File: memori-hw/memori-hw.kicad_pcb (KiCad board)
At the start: 4 copper layers, 2 parts, among them J1 WeAct Studio 2.9" E-Paper Dis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, J2 Seeed Studio Xiao ESP32-C3

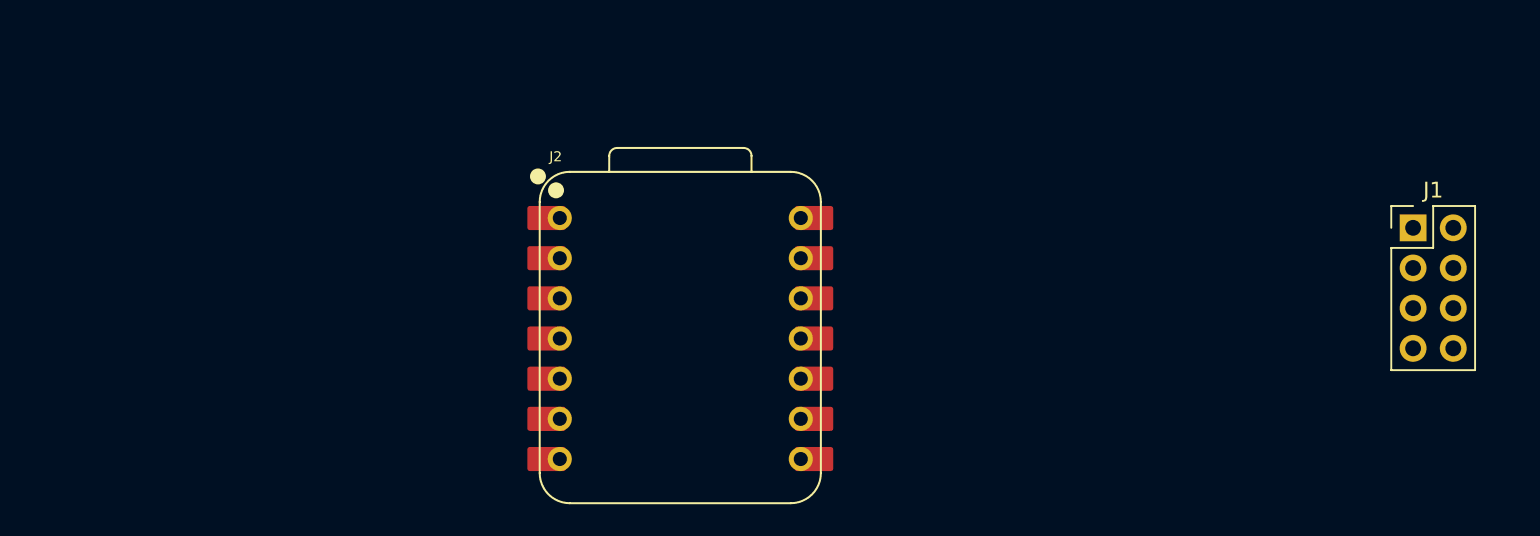
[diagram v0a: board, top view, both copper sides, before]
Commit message: feat(hw): Finished non-battery PCB.
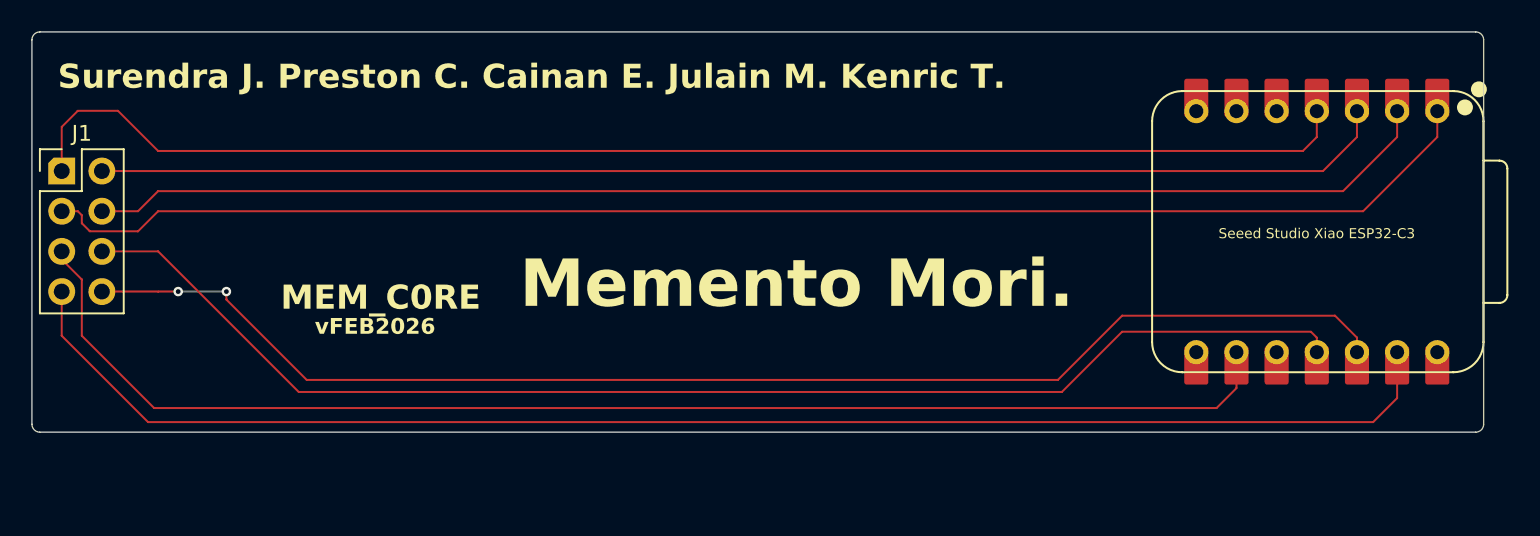
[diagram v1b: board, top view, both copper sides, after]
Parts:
- moved J1 85.5 mm to (95.5, 97.8)
- moved J2 40.7 mm to (174.9, 101.7), turned to -90 degrees
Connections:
- net /GND renamed GND
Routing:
- net GND: track 0.00 -> 92.2 mm
- net /D/C: track 0.00 -> 91.9 mm
- net /BUSY: track 0.00 -> 85.6 mm
- net /CS: track 0.00 -> 85.5 mm
- net /3V3: track 0.00 -> 85.2 mm, vias 0 -> 2
- net /SDA: track 0.00 -> 83.2 mm
- net /SCL: track 0.00 -> 82.7 mm
- net /RES: track 0.00 -> 81.9 mm
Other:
- board outline added: 91.8 x 25.3 mm
- board text added: "MEM_C0RE"
- board text added: "Memento Mori."
- board text added: "Surendra J. Preston C. Cainan E. Julain M. Kenric T."
- board text added: "vFEB2026"
